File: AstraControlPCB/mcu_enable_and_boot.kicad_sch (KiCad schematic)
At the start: 13 parts, among them SW1 TS_Basic_Small, SW2 TS_Basic_Small

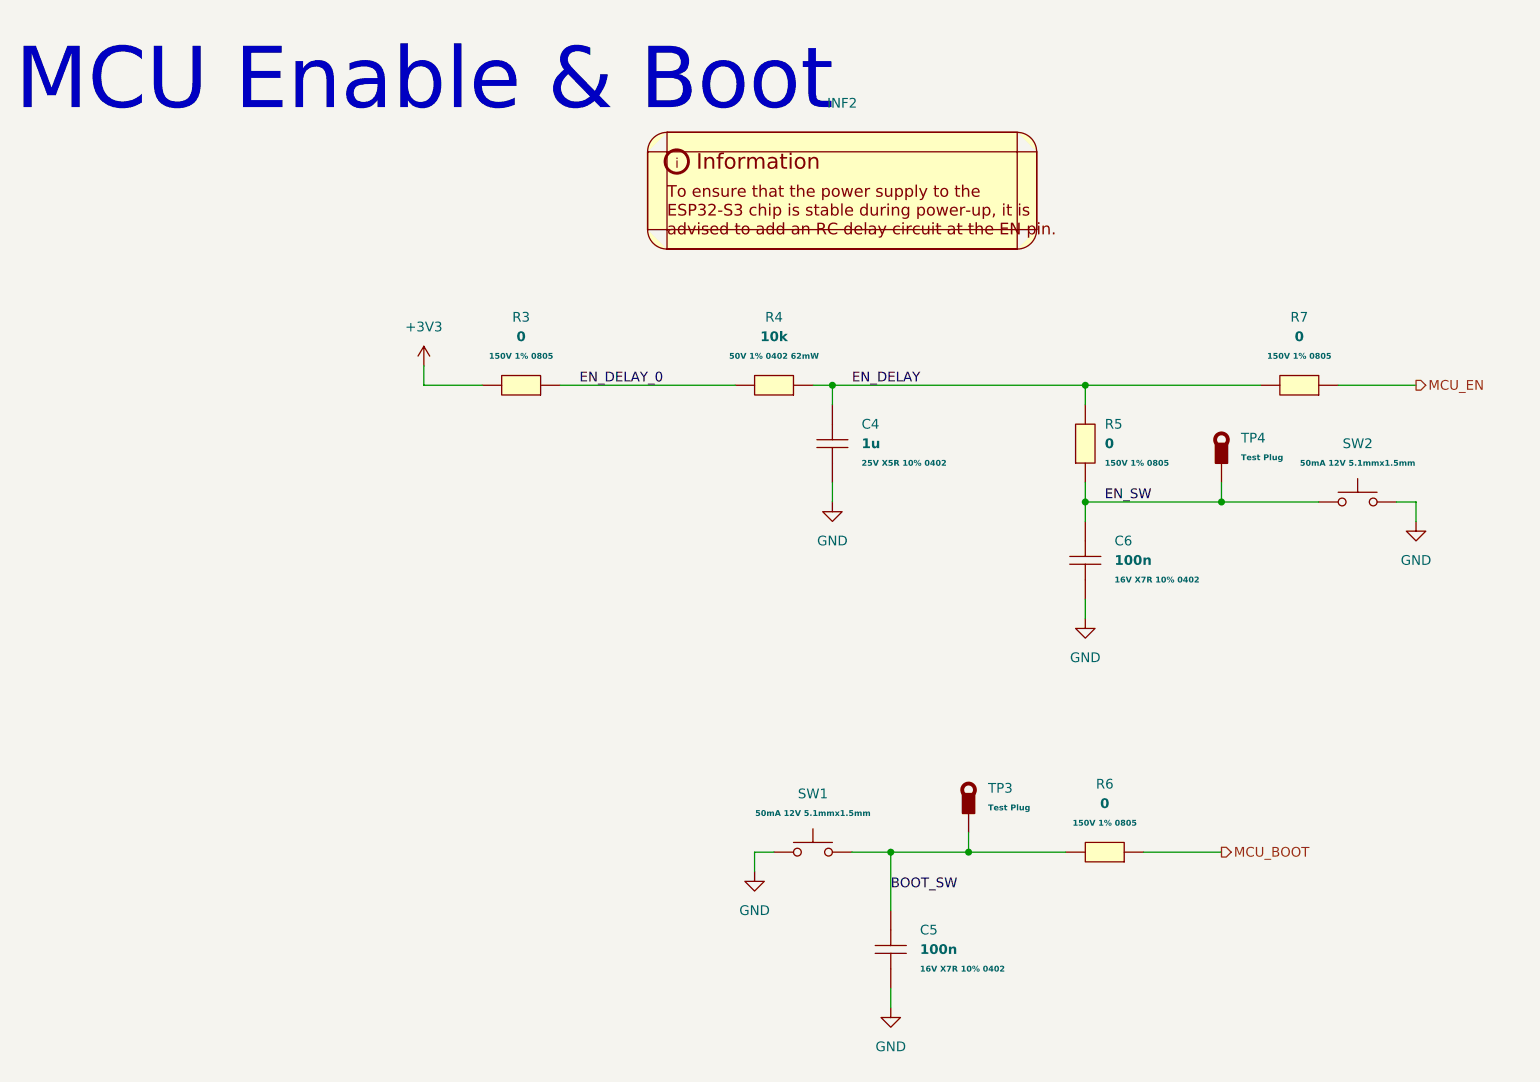
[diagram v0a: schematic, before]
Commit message: update
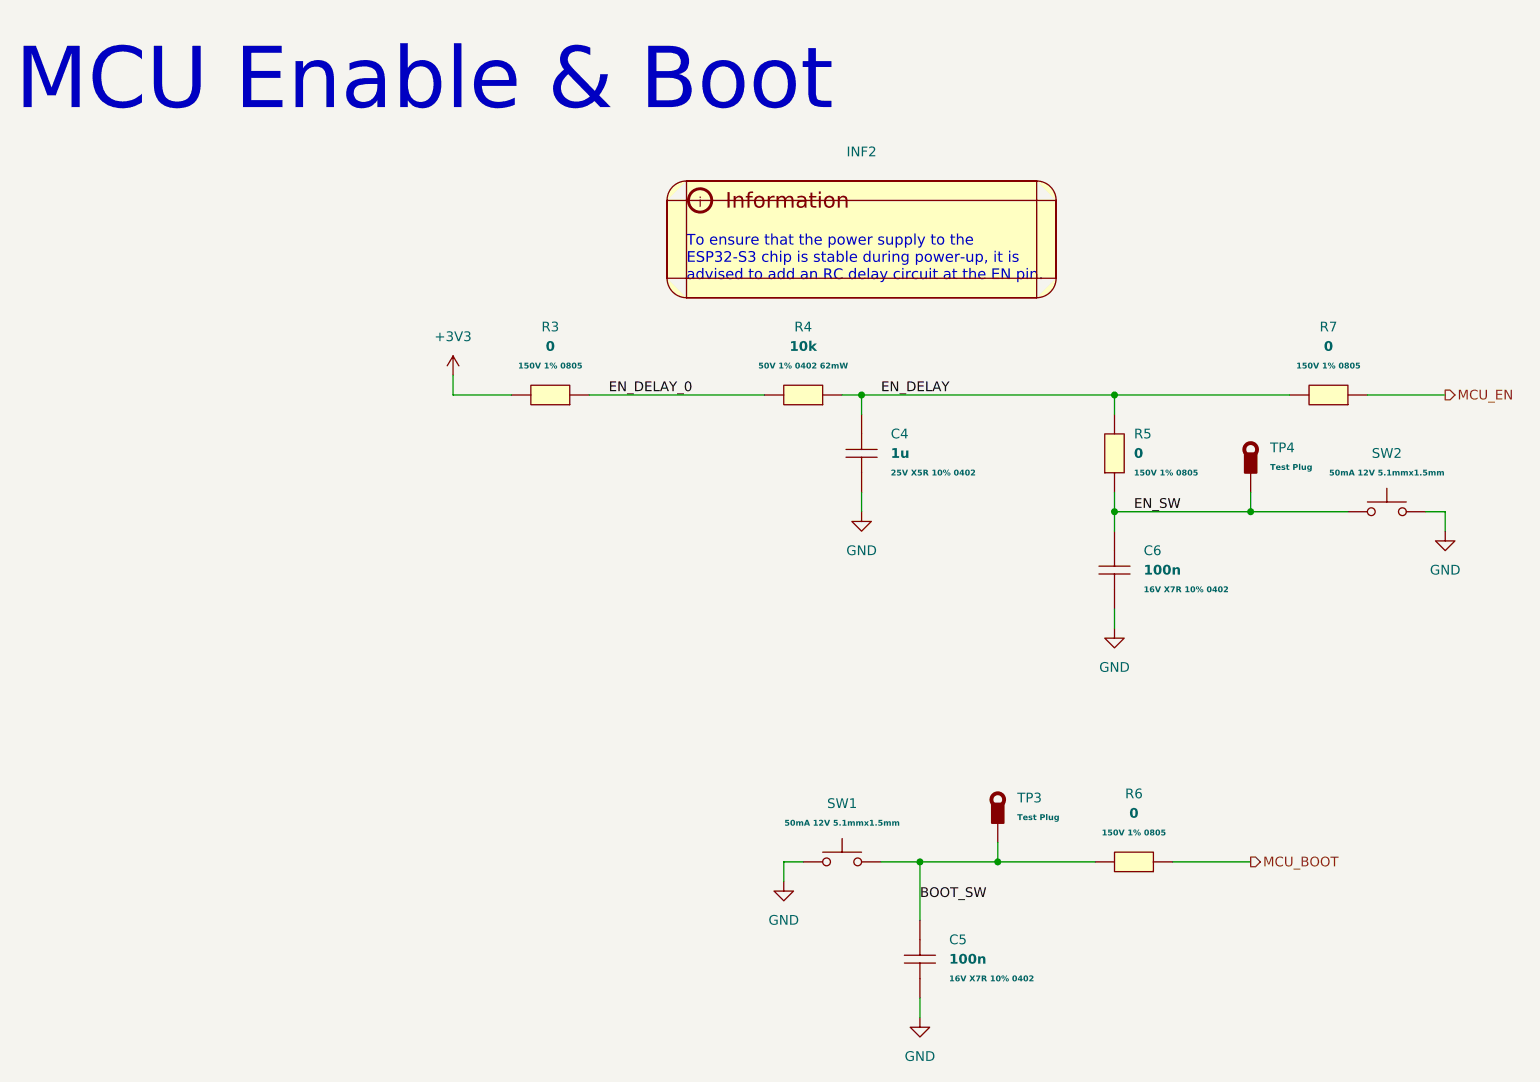
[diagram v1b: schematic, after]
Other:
- note added: "To ensure that the power supply to the ESP32-S3 chip is stable during power-up, it is advised to add an RC delay circuit at the EN pin."
- moved on the sheet: C4, C5, C6, R3, R4, R5, R6, R7, SW1, SW2, TP3, TP4
